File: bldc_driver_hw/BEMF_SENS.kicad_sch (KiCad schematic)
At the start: 4 parts, among them U12 LM397

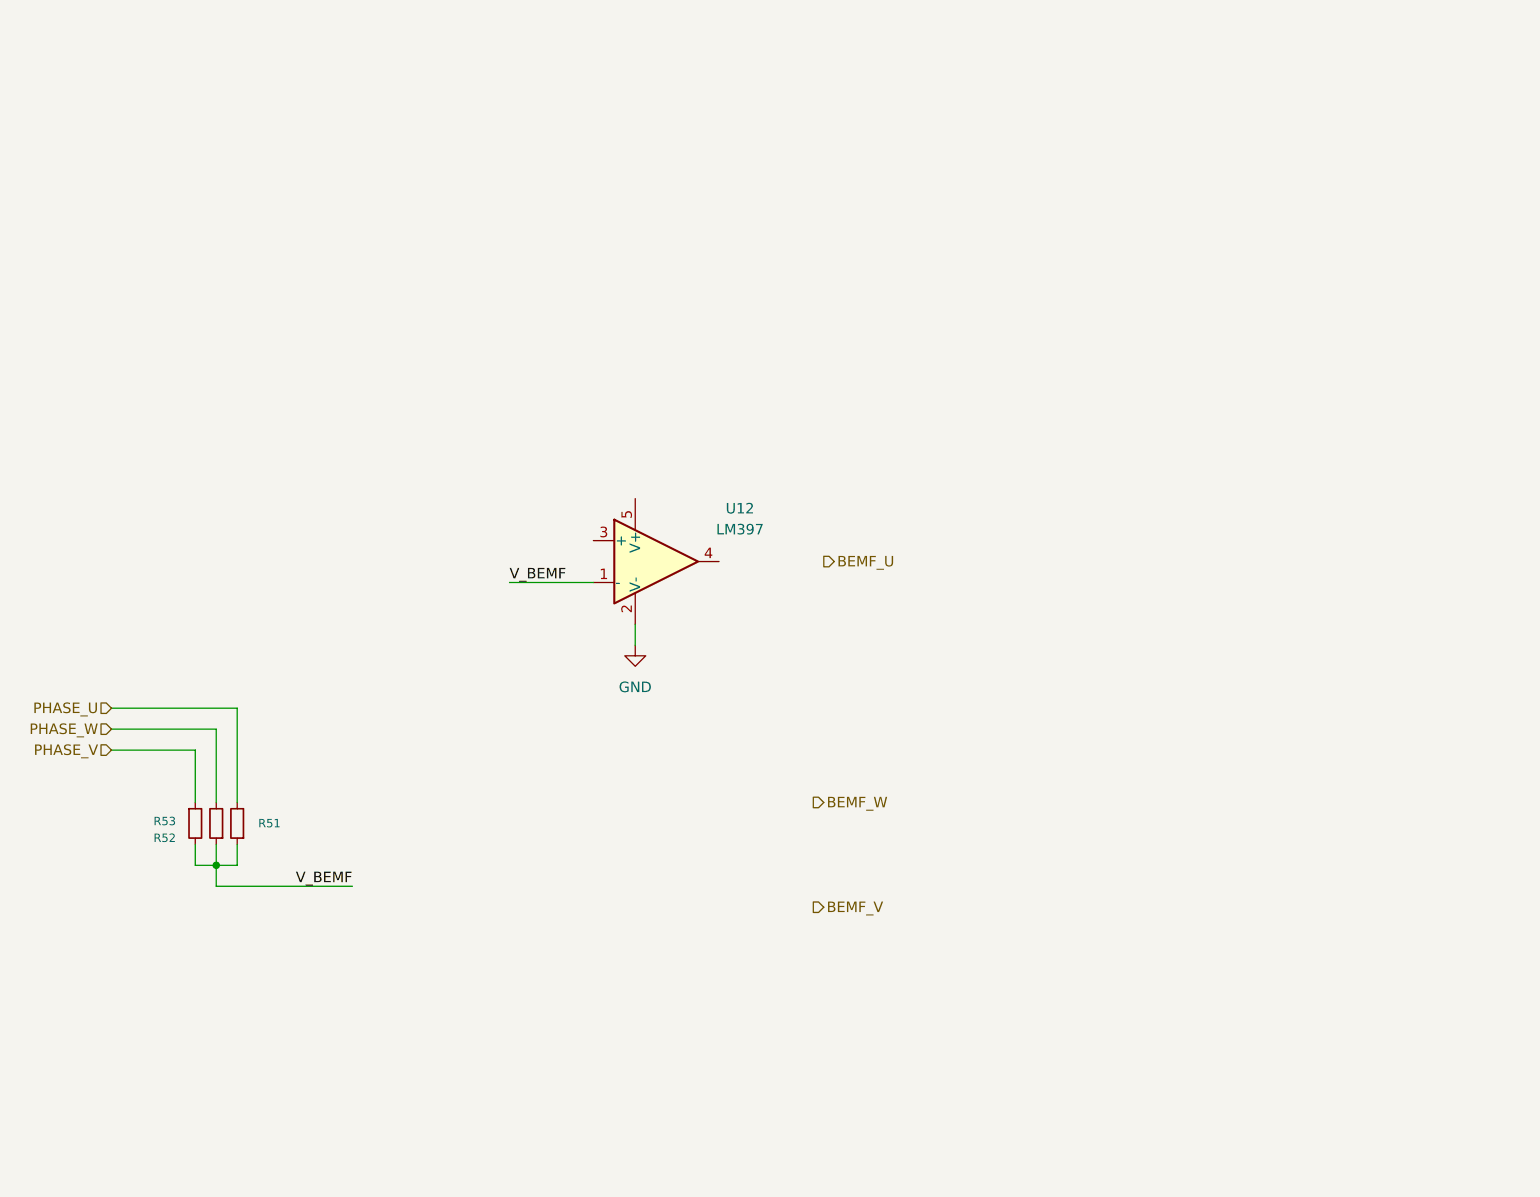
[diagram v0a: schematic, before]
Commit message: wip
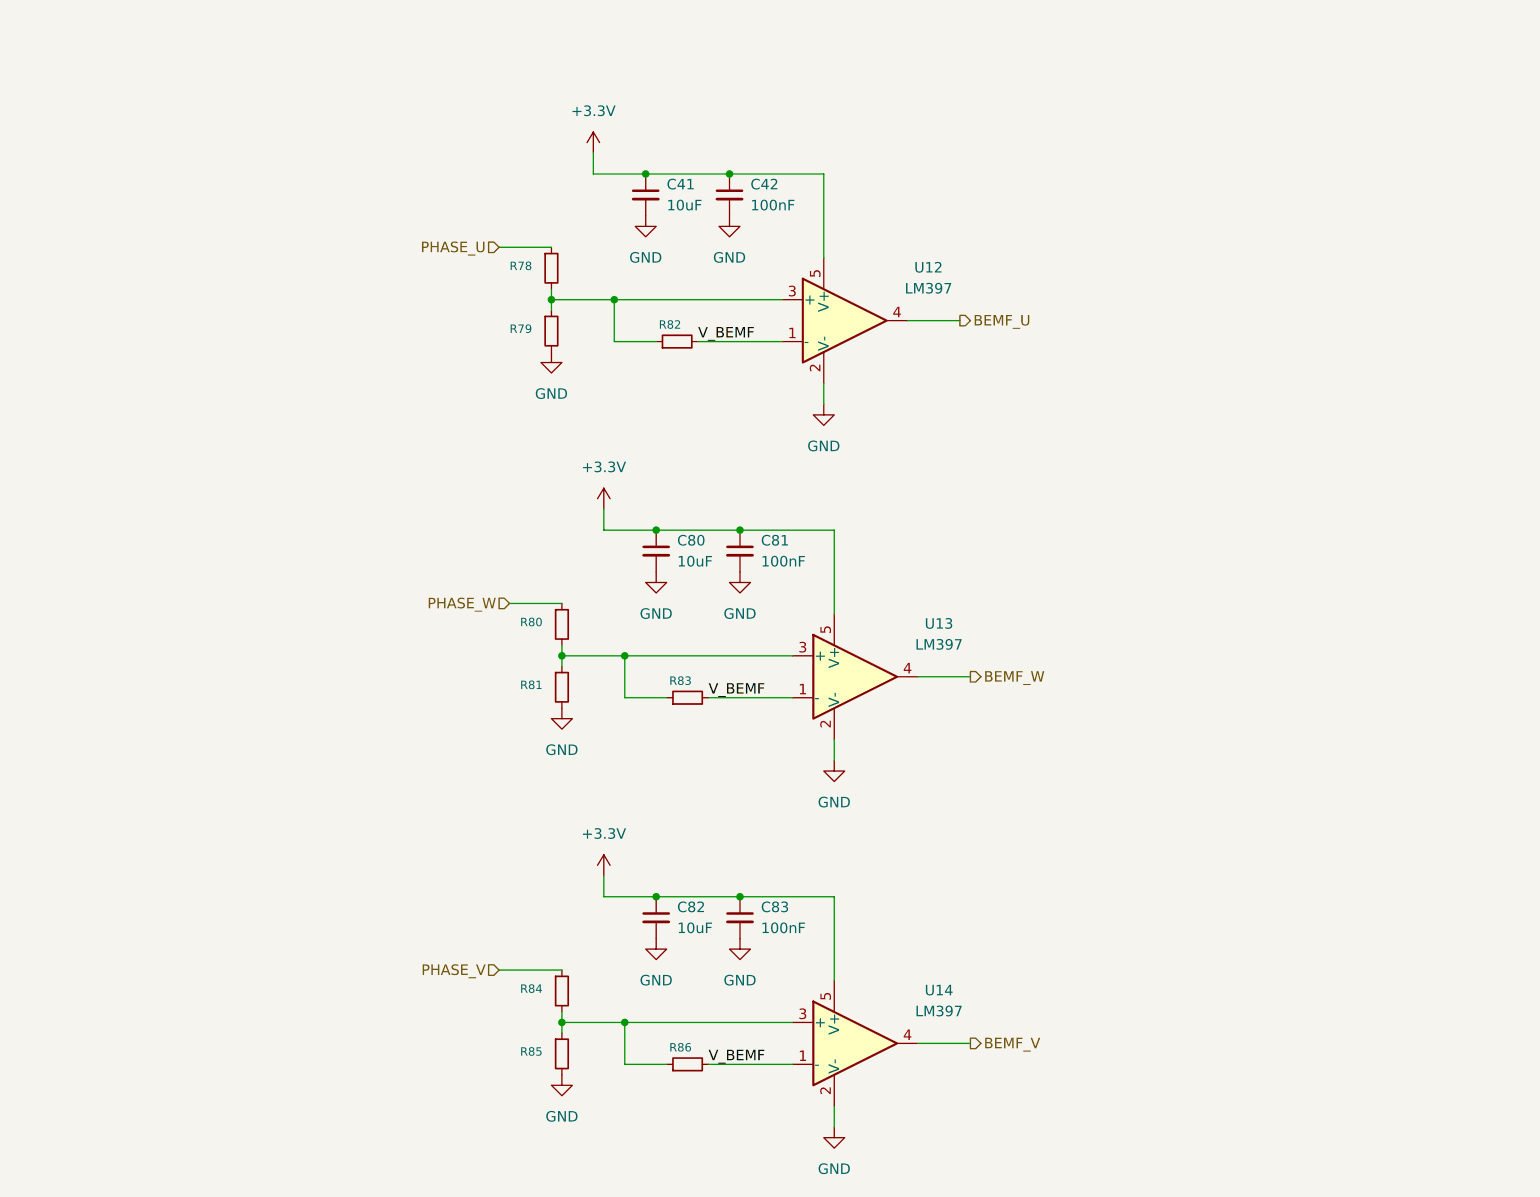
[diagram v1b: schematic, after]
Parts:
- removed R51, R52, R53: R_Small, symbol Device:R_Small
- added C41, C80, C82: 10uF, Capacitor_SMD:C_0805_2012Metric_Pad1.18x1.45mm_HandSolder, symbol Device:C_Small
- added C42, C81, C83: 100nF, Capacitor_SMD:C_0603_1608Metric_Pad1.08x0.95mm_HandSolder, symbol Device:C_Small
- added R78, R79, R80, R81, R82, R83, R84, R85, R86: R_Small, symbol Device:R_Small
- added U13, U14: LM397, Package_TO_SOT_SMD:SOT-23-5, symbol Comparator:LM397
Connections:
- net BEMF_U: now also U12.4
- net BEMF_V: now also U14.4
- net BEMF_W: now also U13.4
- net GND: now also C41.2, C42.2, C80.2, C81.2, C82.2, C83.2, R79.2, R81.2, R85.2, U13.2 (V-), U14.2 (V-)
- net PHASE_U: now also R78.1
- net PHASE_V: now also R84.1
- net PHASE_W: now also R80.1
- net V_BEMF: now also R82.2, R83.2, R86.2, U13.1 (-), U14.1 (-)
- net at U12.3 (+): now also R78.2, R79.1, R82.1
- net +3.3V: now reaches U12.5 (V+)
- net +3.3V: now also C41.1, C42.1, C80.1, C81.1, C82.1, C83.1, U13.5 (V+), U14.5 (V+)
- new net: R80.2, R81.1, R83.1, U13.3 (+)
- new net: R84.2, R85.1, R86.1, U14.3 (+)
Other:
- moved on the sheet: U12

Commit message: schematic finished pcb in progress
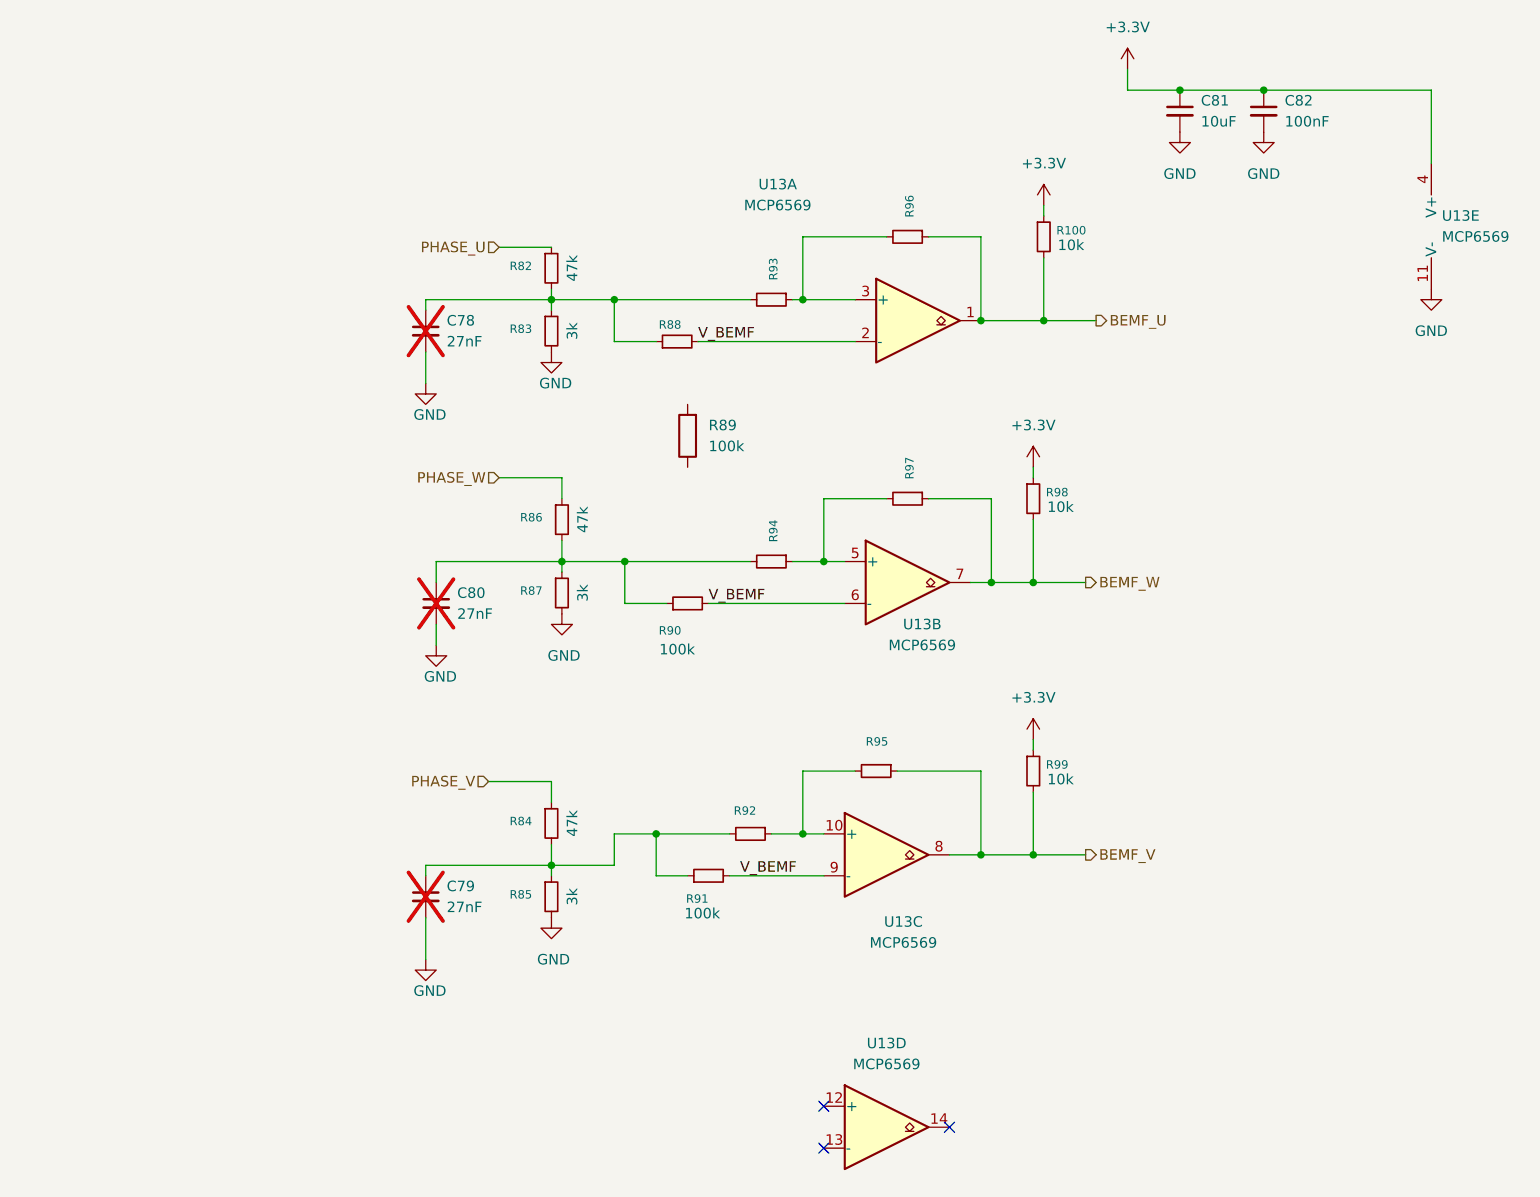
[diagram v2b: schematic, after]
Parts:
- removed C81, C83: 100nF, Capacitor_SMD:C_0603_1608Metric_Pad1.08x0.95mm_HandSolder, symbol Device:C_Small
- removed C82: 10uF, Capacitor_SMD:C_0805_2012Metric_Pad1.18x1.45mm_HandSolder, symbol Device:C_Small
- removed R80, R81: R_Small, symbol Device:R_Small
- removed U12, U13, U14: LM397, Package_TO_SOT_SMD:SOT-23-5, symbol Comparator:LM397
- added C78, C79: 27nF, Capacitor_SMD:C_0603_1608Metric, symbol Device:C_Small
- added R100, R98, R99: 10k, Resistor_SMD:R_0603_1608Metric, symbol Device:R_Small
- added R86: 47k, Resistor_SMD:R_0603_1608Metric, symbol Device:R_Small
- added R87: 3k, Resistor_SMD:R_0603_1608Metric, symbol Device:R_Small
- added R89: 100k, Resistor_SMD:R_0603_1608Metric, symbol Device:R
- added R92, R93, R94, R95, R96, R97: R_Small, Resistor_SMD:R_0603_1608Metric, symbol Device:R_Small
- added U13: MCP6569, Package_SO:SOIC-14_3.9x8.7mm_P1.27mm, symbol Comparator:MCP6569
- C80: value 10uF -> 27nF; footprint Capacitor_SMD:C_0805_2012Metric_Pad1.18x1.45mm_HandSolder -> Capacitor_SMD:C_0603_1608Metric; now not fitted
- R82: renamed from R78; value R_Small -> 47k; footprint (none) -> Resistor_SMD:R_0603_1608Metric
- R83: renamed from R79; value R_Small -> 3k; footprint (none) -> Resistor_SMD:R_0603_1608Metric
- R84: value R_Small -> 47k; footprint (none) -> Resistor_SMD:R_0603_1608Metric
- R85: value R_Small -> 3k; footprint (none) -> Resistor_SMD:R_0603_1608Metric
- R88: renamed from R82; value R_Small -> 100k; footprint (none) -> Resistor_SMD:R_0603_1608Metric
- R90: renamed from R83; value R_Small -> 100k; footprint (none) -> Resistor_SMD:R_0603_1608Metric
- R91: renamed from R86; value R_Small -> 100k; footprint (none) -> Resistor_SMD:R_0603_1608Metric
- renumbered C41 to C81, C42 to C82
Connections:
- net +3.3V: now also R100.1, R98.1, R99.1, U13.4 (V+); no longer C80.1
- net BEMF_U: now also R100.2, R96.1, U13.1
- net BEMF_V: now also R95.1, R99.2, U13.8
- net BEMF_W: now also R97.1, R98.2, U13.7
- net GND: now also C78.2, C79.2, R87.2, U13.11 (V-)
- net PHASE_W: now also R86.1
- net V_BEMF: now also U13.2 (-), U13.6 (-), U13.9 (-)
- net at R82.2, R83.1, R88.1: now also C78.1, R93.2
- net at R90.1: now also C80.1, R86.2, R87.1, R94.2
- net at R84.2, R85.1, R91.1: now also C79.1, R92.2
- new net: R92.1, R95.2, U13.10 (+)
- new net: R94.1, R97.2, U13.5 (+)
- new net: R93.1, R96.2, U13.3 (+)
- no-connect marks 0 -> 3
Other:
- moved on the sheet: C81, C82, R90, R91
